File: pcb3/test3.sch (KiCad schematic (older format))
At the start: 52 parts, among them CON1 BARREL_JACK, CON2 BARREL_JACK, IC1 ATMEGA8A-A, P1 USB_A, SW1 SW_PUSH

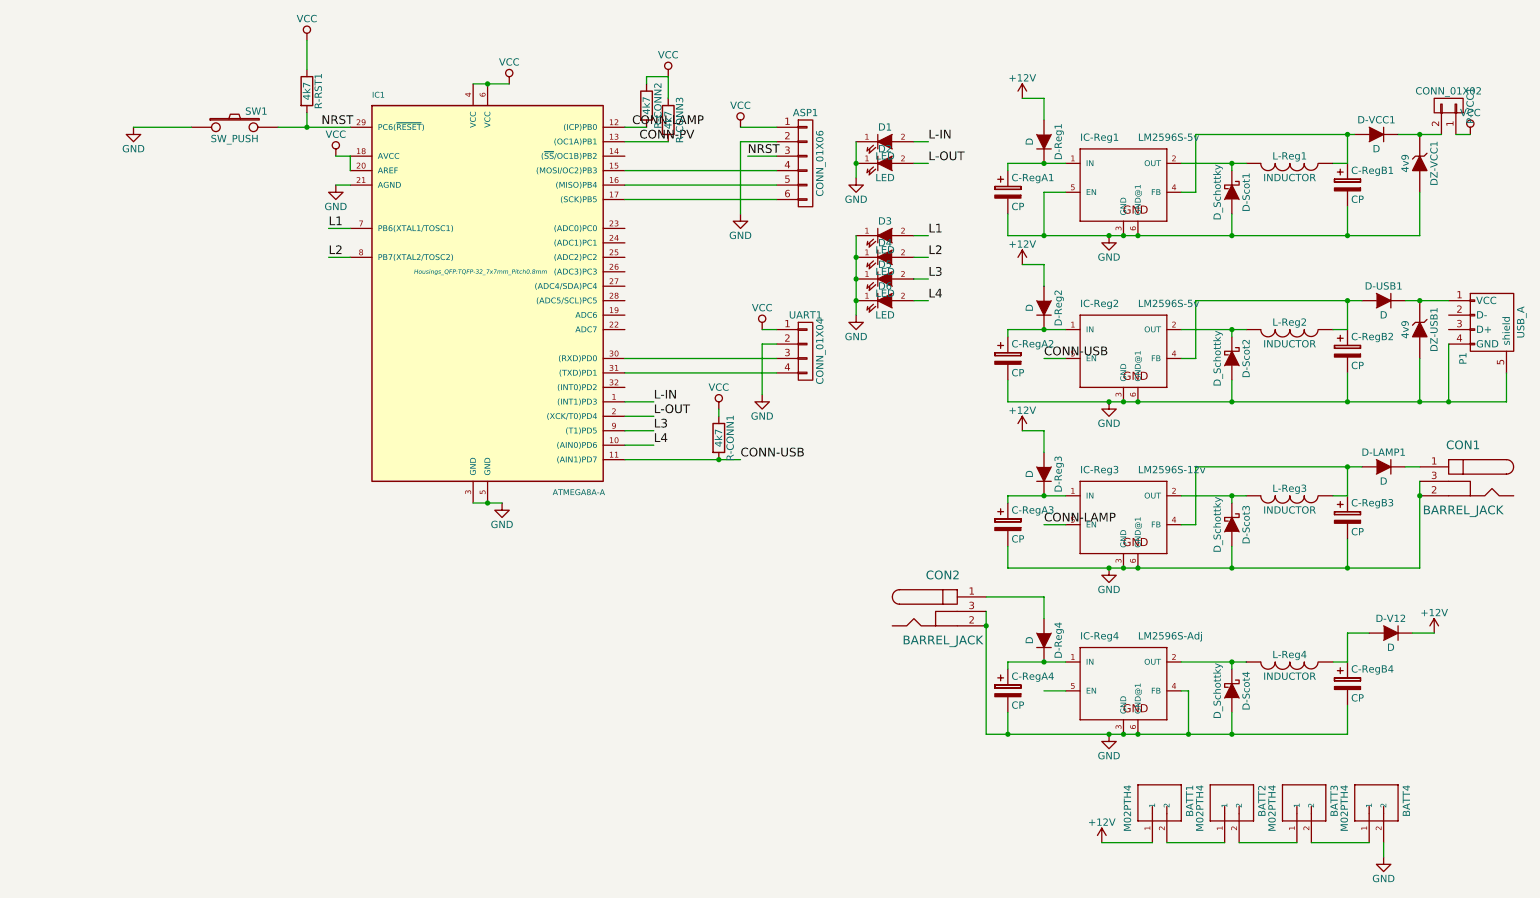
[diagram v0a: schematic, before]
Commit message: belum apply revisi
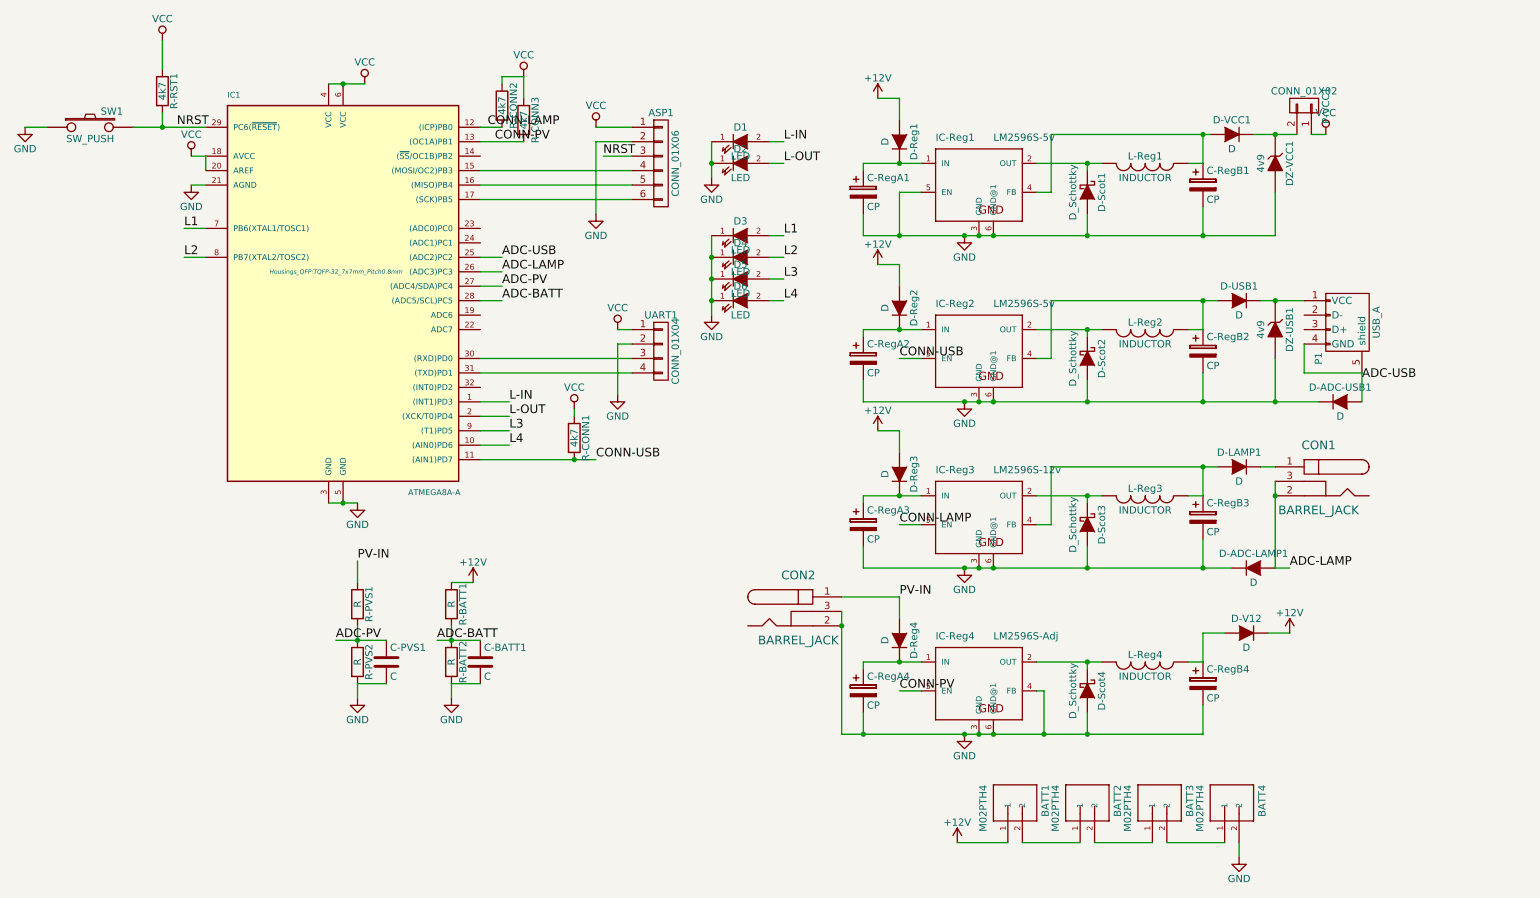
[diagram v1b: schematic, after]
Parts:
- added C-BATT1, C-PVS1: C, Capacitors_ThroughHole:C_Rect_L7_W2_P5, symbol C
- added D-ADC-LAMP1, D-ADC-USB1: D, Diodes_ThroughHole:Diode_DO-35_SOD27_Horizontal_RM10, symbol D
- added R-BATT1, R-BATT2, R-PVS1, R-PVS2: R, Resistors_ThroughHole:Resistor_Horizontal_RM10mm, symbol R
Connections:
- net +12V: now also R-BATT1.1
- net CONN-PV: now also IC-Reg4.5 (EN)
- net GND: now also C-BATT1.2, C-PVS1.2, D-ADC-LAMP1.1 (K), D-ADC-USB1.1 (K), R-BATT2.2, R-PVS2.2; no longer CON1.2, CON1.3, P1.4 (GND), P1.5 (shield)
- net ADC-USB: now reaches IC1.25 ((ADC2)PC2)
- net ADC-USB: now also P1.4 (GND), P1.5 (shield), D-ADC-USB1.2 (A)
- net ADC-LAMP: now reaches IC1.26 ((ADC3)PC3)
- net ADC-LAMP: now also CON1.2, CON1.3, D-ADC-LAMP1.2 (A)
- net ADC-PV: now reaches IC1.27 ((ADC4/SDA)PC4)
- net ADC-PV: now also C-PVS1.1, R-PVS1.2, R-PVS2.1
- net ADC-BATT: now reaches IC1.28 ((ADC5/SCL)PC5)
- net ADC-BATT: now also C-BATT1.1, R-BATT1.2, R-BATT2.1
- net PV-IN: now reaches CON2.1, D-Reg4.2 (A)
- net PV-IN: now also R-PVS1.1
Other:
- moved on the sheet: ASP1, BATT1, BATT2, BATT3, BATT4, C-RegA1, C-RegA2, C-RegA3, C-RegA4, C-RegB1, C-RegB2, C-RegB3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

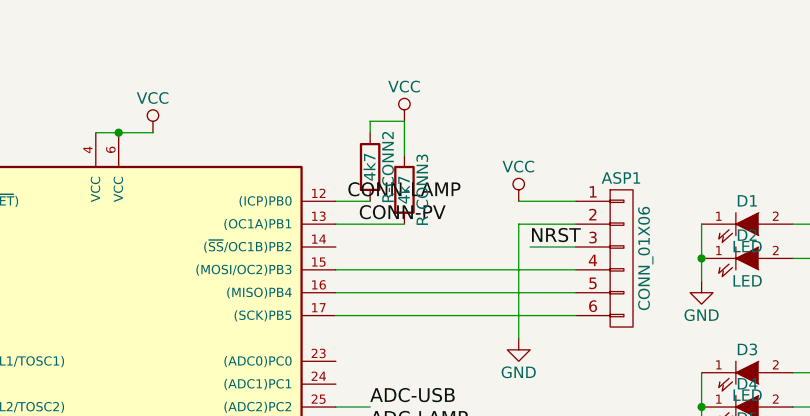
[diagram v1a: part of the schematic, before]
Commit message: ready to build
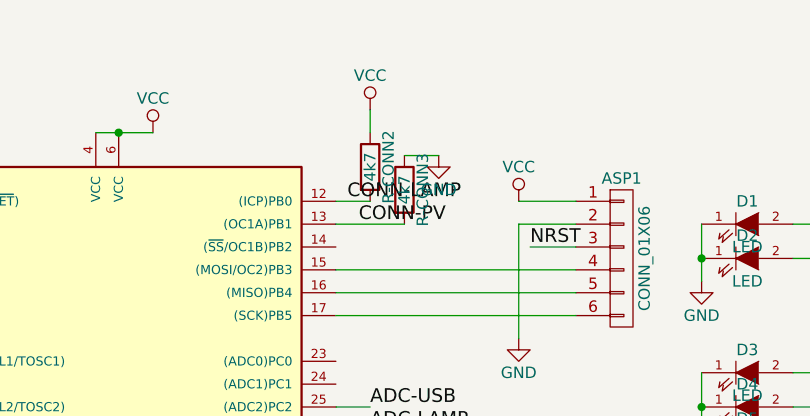
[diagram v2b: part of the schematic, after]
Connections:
- net GND: now also R-CONN3.1
- net VCC: no longer R-CONN3.1
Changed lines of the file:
@@
 L VCC #PWR025
 U 1 1 56304D29
-P 4100 900
-F 0 "#PWR025" H 4100 750 50  0001 C CNN
-F 1 "VCC" H 4100 1050 50  0000 C CNN
-F 2 "" H 4100 900 60  0000 C CNN
-F 3 "" H 4100 900 60  0000 C CNN
-	1    4100 900
+P 3950 850
+F 0 "#PWR025" H 3950 700 50  0001 C CNN
+F 1 "VCC" H 3950 1000 50  0000 C CNN
+F 2 "" H 3950 850 60  0000 C CNN
+F 3 "" H 3950 850 60  0000 C CNN
+	1    3950 850
 	1    0    0    -1
 $EndComp
@@
 	3800 1350 4100 1350
 Wire Wire Line
-	3950 950  3950 900
-Wire Wire Line
-	3950 900  4100 900
-Wire Wire Line
-	4100 900  4100 1050
-Wire Wire Line
 	6300 4500 6700 4500
 Wire Wire Line
@@
 Text Label 3950 2150 0    60   ~ 0
 ADC-USB
+$Comp
+L GND #PWR?
+U 1 1 563787DD
+P 4250 1050
+F 0 "#PWR?" H 4250 800 50  0001 C CNN
+F 1 "GND" H 4250 900 50  0000 C CNN
+F 2 "" H 4250 1050 60  0000 C CNN
+F 3 "" H 4250 1050 60  0000 C CNN
+	1    4250 1050
+	1    0    0    -1
+$EndComp
+Wire Wire Line
+	4250 1050 4100 1050
+Wire Wire Line
+	3950 850  3950 950
 $EndSCHEMATC
